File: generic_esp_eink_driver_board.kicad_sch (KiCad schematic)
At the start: 53 parts, among them IC1 TPS7A0233PDBVR, IC2 MAX17260SETD+T, J1 USB_C_Receptacle_USB2.0_16P, J2 S2B-PH-SM4-TB, J3 Conn_01x04, Q1 AO3400A, U1 USBLC6-2SC6, U2 BQ24040DSQR, U3 ESP32-S3-WROOM-1, U4 FPC24

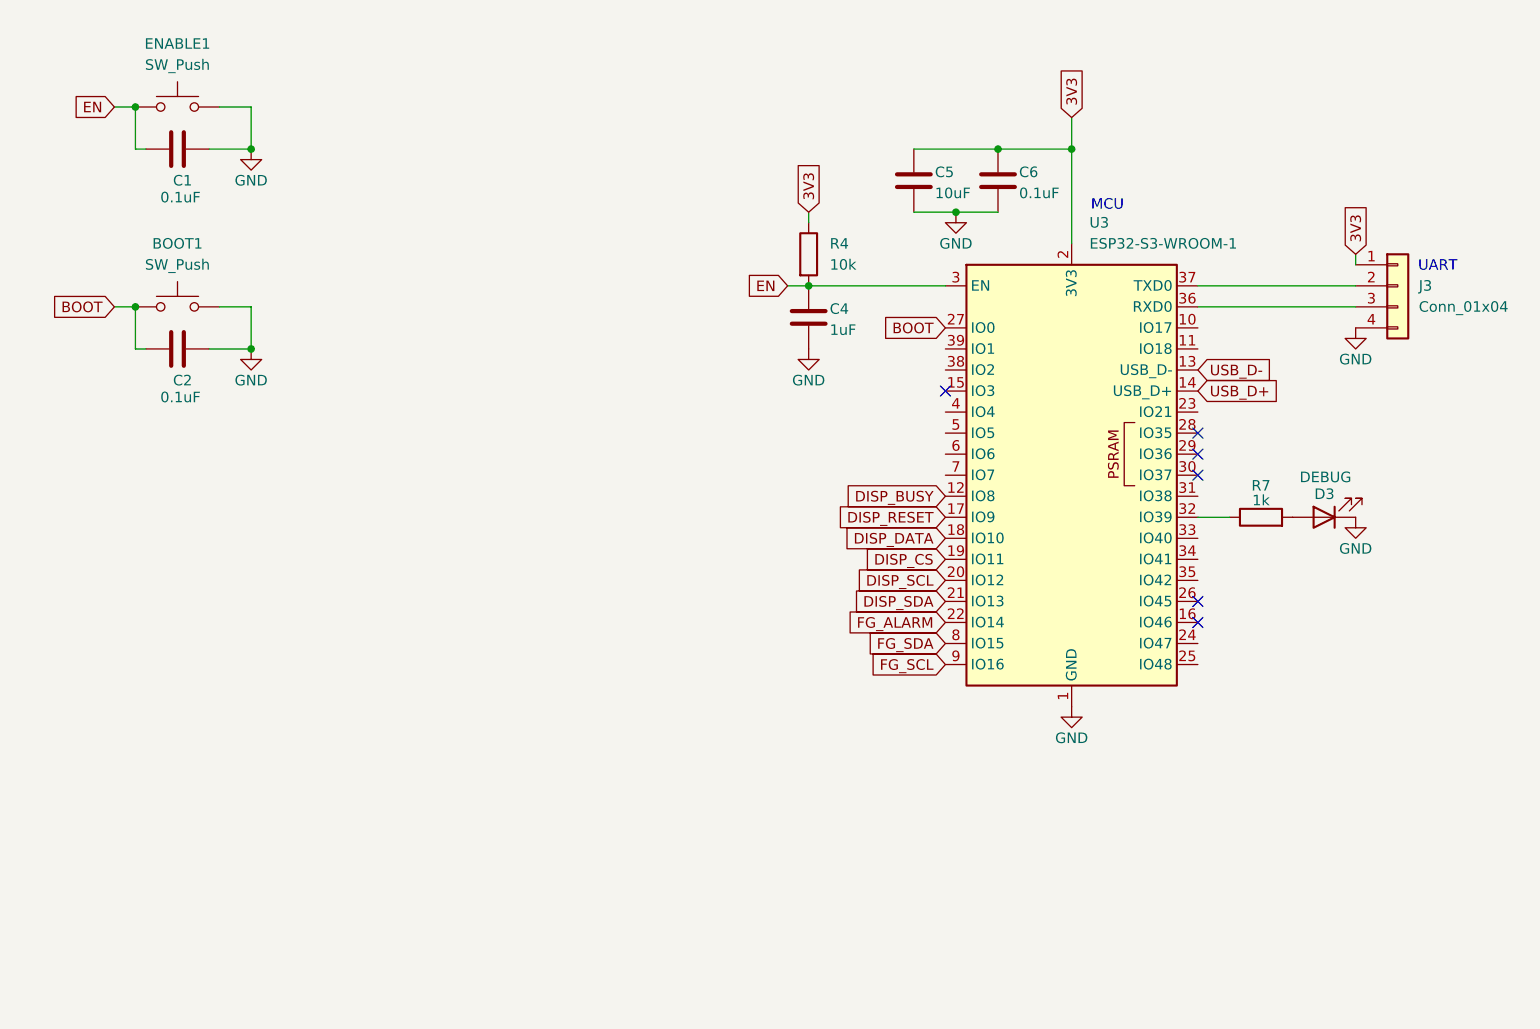
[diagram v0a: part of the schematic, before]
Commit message: re-placement
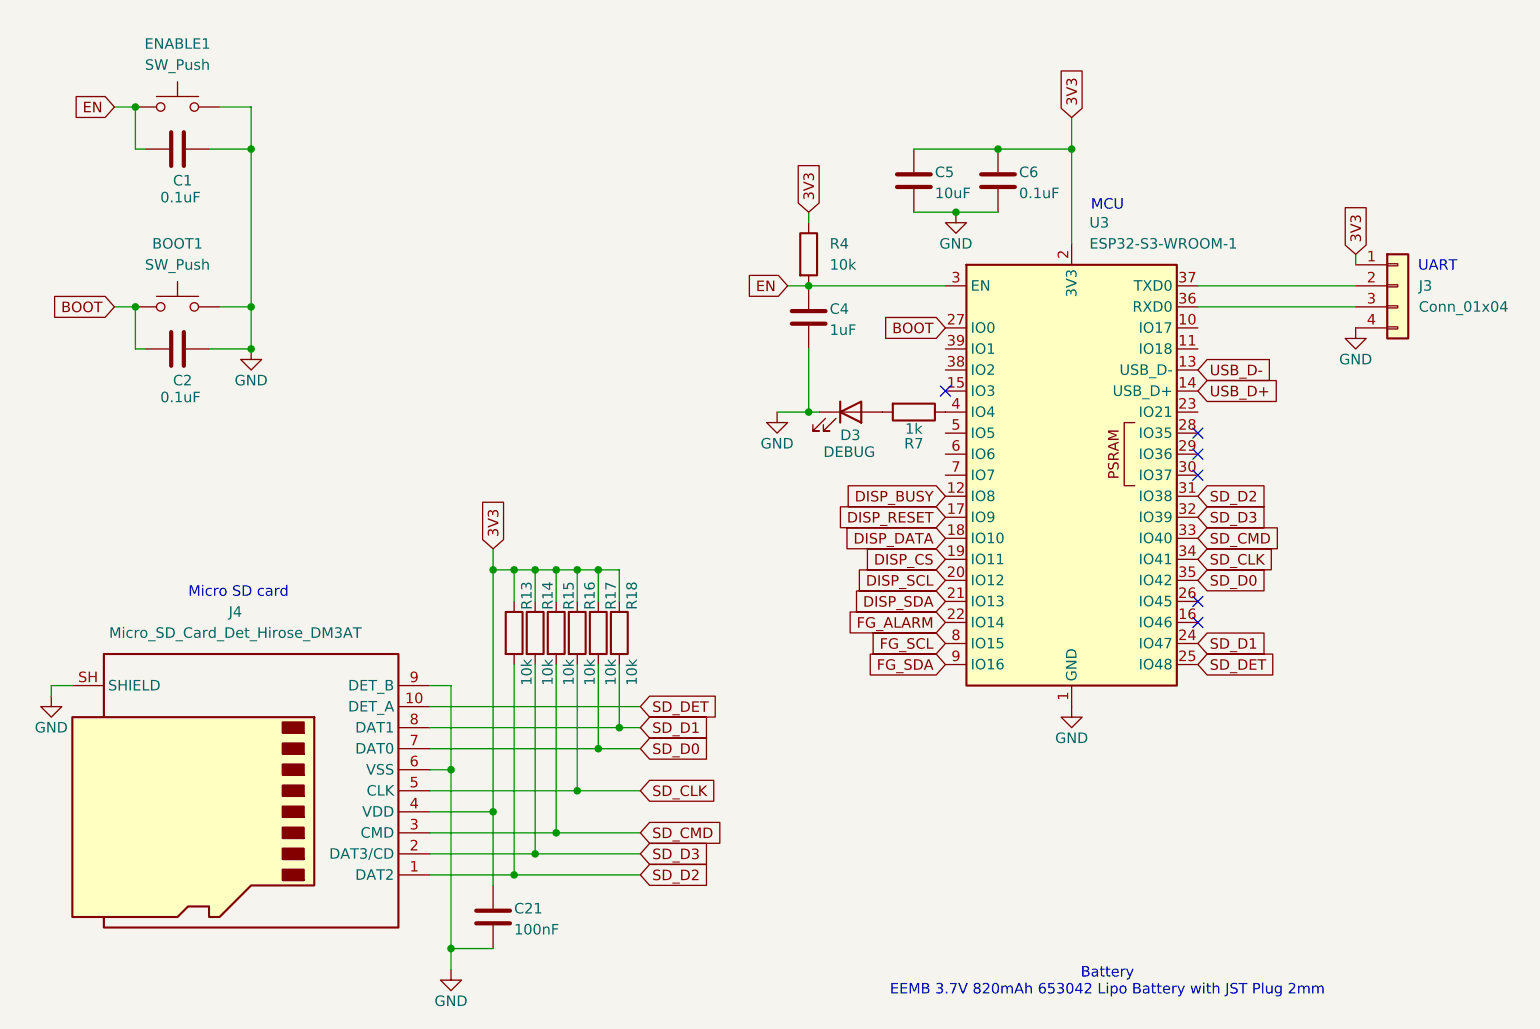
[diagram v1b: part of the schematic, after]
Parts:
- added C21: 100nF, Capacitor_SMD:C_0805_2012Metric_Pad1.18x1.45mm_HandSolder, symbol Device:C
- added J4: Micro_SD_Card_Det_Hirose_DM3AT, Connector_Card:microSD_HC_Hirose_DM3AT-SF-PEJM5, symbol Connector:Micro_SD_Card_Det_Hirose_DM3AT
- added R13, R14, R15, R16, R17, R18: 10k, Resistor_SMD:R_0805_2012Metric_Pad1.20x1.40mm_HandSolder, symbol Device:R
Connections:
- net 3V3: now also C21.1, J4.4 (VDD), R13.1, R14.1, R15.1, R16.1, R17.1, R18.1
- net FG_SCL: now also U3.8 (IO15); no longer U3.9 (IO16)
- net FG_SDA: now also U3.9 (IO16); no longer U3.8 (IO15)
- net GND: now also C21.2, J4.6 (VSS), J4.9 (DET_B), J4.SH (SHIELD)
- net SD_D1: now reaches U3.24 (IO47)
- net SD_D1: now also J4.8 (DAT1), R18.2
- net SD_DET: now reaches U3.25 (IO48)
- net SD_DET: now also J4.10 (DET_A)
- net SD_D2: now reaches U3.31 (IO38)
- net SD_D2: now also J4.1 (DAT2), R13.2
- net at R7.1: now also U3.4 (IO4); no longer U3.32 (IO39)
- net SD_CMD: now reaches U3.33 (IO40)
- net SD_CMD: now also J4.3 (CMD), R15.2
- net SD_CLK: now reaches U3.34 (IO41)
- net SD_CLK: now also J4.5 (CLK), R16.2
- net SD_D0: now reaches U3.35 (IO42)
- net SD_D0: now also J4.7 (DAT0), R17.2
- new net SD_D3: J4.2 (DAT3/CD), R14.2, U3.32 (IO39)
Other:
- note added: "Battery EEMB 3.7V 820mAh 653042 Lipo Battery with JST Plug 2mm"
- note added: "Micro SD card"
- moved on the sheet: D3, R7
